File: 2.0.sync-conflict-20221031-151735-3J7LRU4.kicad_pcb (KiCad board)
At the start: 2 copper layers, 38.1 x 50 mm, 26 parts, among them J1 MK-12C02

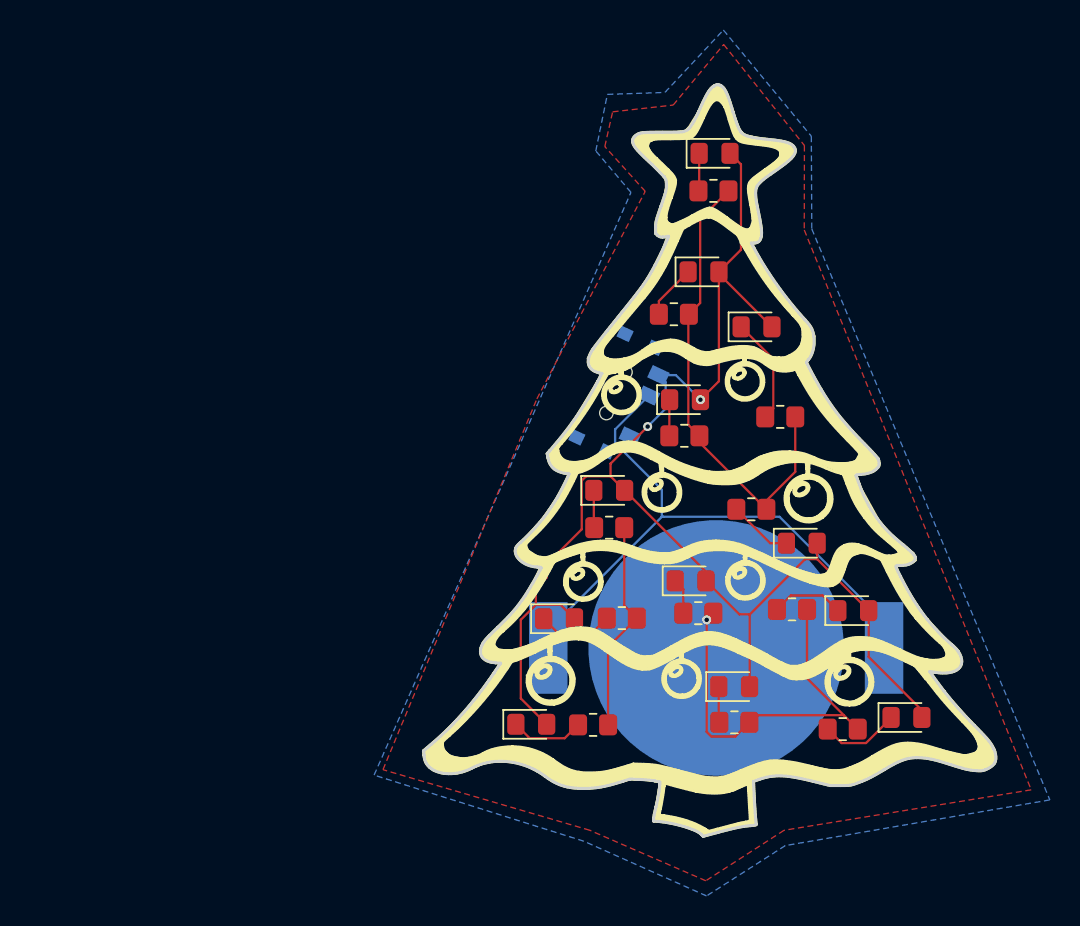
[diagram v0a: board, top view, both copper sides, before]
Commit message: Fixed PCB
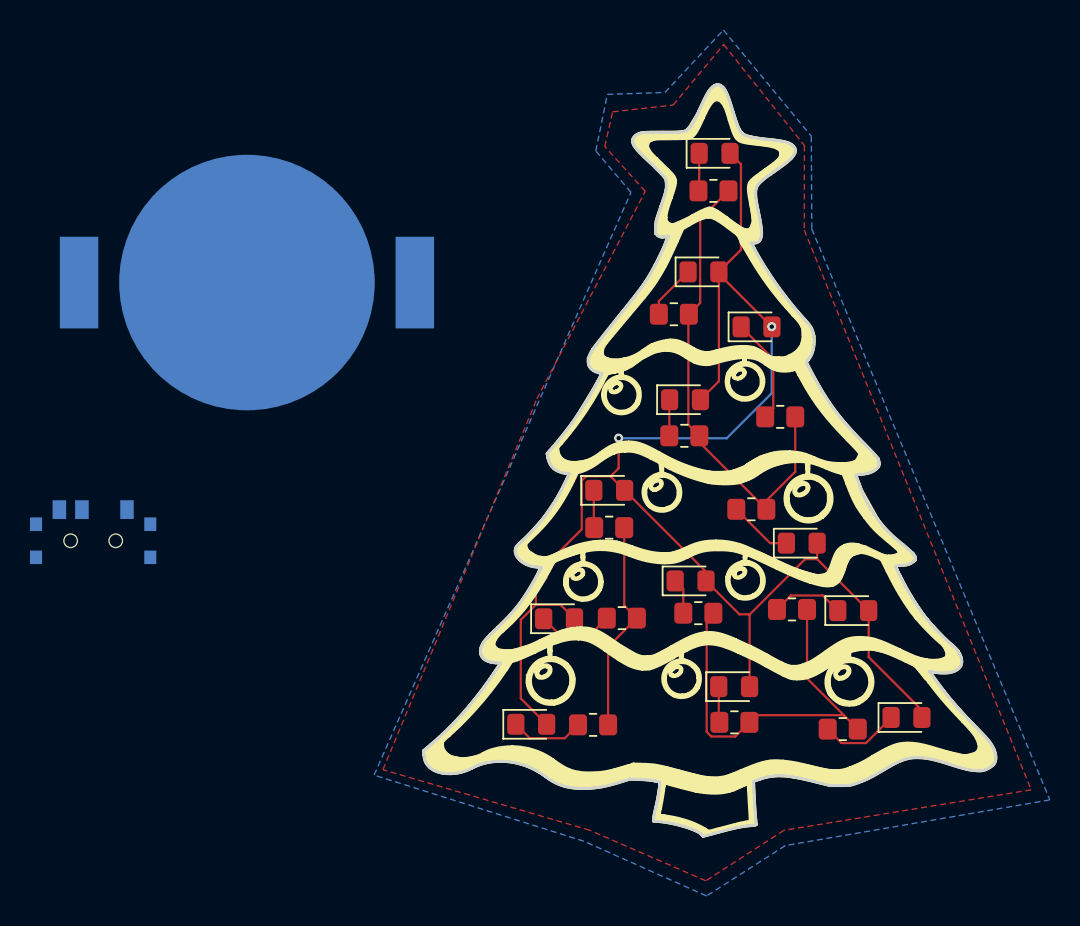
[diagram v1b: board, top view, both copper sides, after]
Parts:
- moved BT1 39.6 mm to (149.6, 89.8)
- moved J1 36.2 mm to (139.3, 107.0), turned to 180 degrees
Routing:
- net Net-(BT1-Pad1): track 43.6 -> 0.00 mm
- net Net-(D1-Pad2): track 97.0 -> 103.8 mm
- net GND: vias 1 -> 0
